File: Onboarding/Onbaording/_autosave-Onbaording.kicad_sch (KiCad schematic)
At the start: 3 parts, among them J1 Screw_Terminal_2x2.54

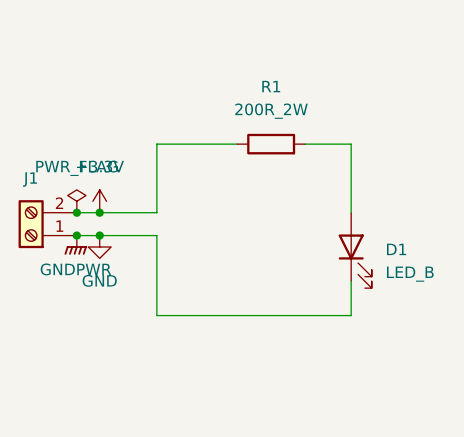
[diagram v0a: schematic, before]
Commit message: more instructions
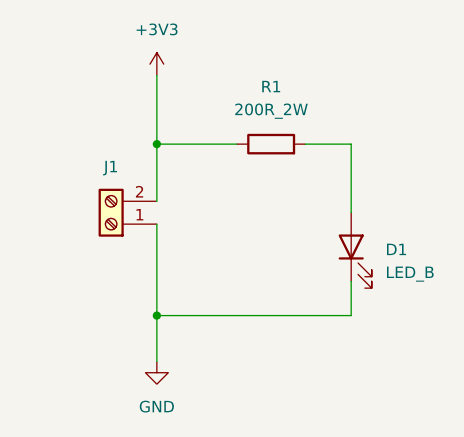
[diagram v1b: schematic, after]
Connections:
- net +3.3V renamed +3V3
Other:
- moved on the sheet: J1
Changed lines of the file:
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@@
 	(paper "A5")
 	(junction
-		(at 53.34 43.18)
+		(at 59.69 33.02)
 		(diameter 0)
 		(color 0 0 0 0)
 	)
 	(junction
-		(at 50.8 40.64)
+		(at 59.69 52.07)
 		(diameter 0)
 		(color 0 0 0 0)
 	)
-	(junction
-		(at 50.8 43.18)
-		(diameter 0)
-		(color 0 0 0 0)
-	)
-	(junction
-		(at 53.34 40.64)
-		(diameter 0)
-		(color 0 0 0 0)
-	)
 	(wire
 		(pts
@@
 	(wire
 		(pts
-			(xy 53.34 40.64) (xy 59.69 40.64)
+			(xy 59.69 41.91) (xy 59.69 52.07)
 		)
 		(stroke
@@
 	(wire
 		(pts
-			(xy 59.69 40.64) (xy 59.69 33.02)
-		)
-		(stroke
-			(width 0)
-			(type default)
-		)
-	)
-	(wire
-		(pts
-			(xy 59.69 43.18) (xy 59.69 52.07)
-		)
-		(stroke
-			(width 0)
-			(type default)
-		)
-	)
-	(wire
-		(pts
 			(xy 59.69 52.07) (xy 81.28 52.07)
 		)
@@
 	(wire
 		(pts
-			(xy 50.8 40.64) (xy 53.34 40.64)
-		)
-		(stroke
-			(width 0)
-			(type default)
-		)
-	)
-	(wire
-		(pts
-			(xy 53.34 43.18) (xy 59.69 43.18)
+			(xy 59.69 33.02) (xy 59.69 39.37)
 		)
 		(stroke
@@
 	(wire
 		(pts
-			(xy 50.8 43.18) (xy 53.34 43.18)
+			(xy 59.69 25.4) (xy 59.69 33.02)
+		)
+		(stroke
+			(width 0)
+			(type default)
+		)
+	)
+	(wire
+		(pts
+			(xy 59.69 57.15) (xy 59.69 52.07)
 		)
 		(stroke
@@
 			(width 0)
 			(type default)
-		)
-	)
-	(symbol
-		(lib_id "power:GNDPWR")
-		(at 50.8 43.18 0)
-		(unit 1)
-		(exclude_from_sim no)
-		(in_bom yes)
-		(on_board yes)
-		(dnp no)
-		(fields_autoplaced yes)
-		(property "Reference" "#PWR03"
-			(at 50.8 48.26 0)
-			(effects
-				(font
-					(size 1.27 1.27)
-				)
-				(hide yes)
-			)
-		)
-		(property "Value" "GNDPWR"
-			(at 50.673 46.99 0)
-			(effects
-				(font
-					(size 1.27 1.27)
-				)
-			)
-		)
-		(property "Footprint" ""
-			(at 50.8 44.45 0)
-			(effects
-				(font
-					(size 1.27 1.27)
-				)
-				(hide yes)
-			)
-		)
-		(property "Datasheet" ""
-			(at 50.8 44.45 0)
-			(effects
-				(font
-					(size 1.27 1.27)
-				)
-				(hide yes)
-			)
-		)
-		(property "Description" "Power symbol creates a global label with name \"GNDPWR\" , global ground"
-			(at 50.8 43.18 0)
-			(effects
-				(font
-					(size 1.27 1.27)
-				)
-				(hide yes)
-			)
-		)
-		(pin "1"
-		)
-		(instances
-			(project ""
-				(path "/e318a63f-e1fd-4a3a-bd56-00f9b3552079"
-					(reference "#PWR03")
-					(unit 1)
-				)
-			)
 		)
 	)
@@
 	(symbol
 		(lib_id "power:GND")
-		(at 53.34 43.18 0)
+		(at 59.69 57.15 0)
 		(unit 1)
 		(exclude_from_sim no)
@@
 		(fields_autoplaced yes)
 		(property "Reference" "#PWR01"
-			(at 53.34 49.53 0)
+			(at 59.69 63.5 0)
 			(effects
 				(font
@@
 		)
 		(property "Value" "GND"
-			(at 53.34 48.26 0)
+			(at 59.69 62.23 0)
 			(effects
 				(font
@@
 		)
 		(property "Footprint" ""
-			(at 53.34 43.18 0)
+			(at 59.69 57.15 0)
 			(effects
 				(font
@@
 		)
 		(property "Datasheet" ""
-			(at 53.34 43.18 0)
+			(at 59.69 57.15 0)
 			(effects
 				(font
@@
 		)
 		(property "Description" "Power symbol creates a global label with name \"GND\" , ground"
-			(at 53.34 43.18 0)
+			(at 59.69 57.15 0)
 			(effects
 				(font
@@
 		)
 		(instances
-			(project "Onbaording"
+			(project ""
 				(path "/e318a63f-e1fd-4a3a-bd56-00f9b3552079"
 					(reference "#PWR01")
@@
 	)
 	(symbol
-		(lib_id "power:PWR_FLAG")
-		(at 50.8 40.64 0)
+		(lib_id "power:+3V3")
+		(at 59.69 25.4 0)
 		(unit 1)
 		(exclude_from_sim no)
@@
 		(dnp no)
 		(fields_autoplaced yes)
-		(property "Reference" "#FLG01"
-			(at 50.8 38.735 0)
-			(effects
-				(font
-					(size 1.27 1.27)
-				)
-				(hide yes)
-			)
-		)
-		(property "Value" "PWR_FLAG"
-			(at 50.8 35.56 0)
+		(property "Reference" "#PWR02"
+			(at 59.69 29.21 0)
+			(effects
+				(font
+					(size 1.27 1.27)
+				)
+				(hide yes)
+			)
+		)
+		(property "Value" "+3V3"
+			(at 59.69 20.32 0)
 			(effects
 				(font
@@
 		)
 		(property "Footprint" ""
-			(at 50.8 40.64 0)
-			(effects
-				(font
-					(size 1.27 1.27)
-				)
-				(hide yes)
-			)
-		)
-		(property "Datasheet" "~"
-			(at 50.8 40.64 0)
-			(effects
-				(font
-					(size 1.27 1.27)
-				)
-				(hide yes)
-			)
-		)
-		(property "Description" "Special symbol for telling ERC where power comes from"
-			(at 50.8 40.64 0)
+			(at 59.69 25.4 0)
+			(effects
+				(font
+					(size 1.27 1.27)
+				)
+				(hide yes)
+			)
+		)
+		(property "Datasheet" ""
+			(at 59.69 25.4 0)
+			(effects
+				(font
+					(size 1.27 1.27)
+				)
+				(hide yes)
+			)
+		)
+		(property "Description" "Power symbol creates a global label with name \"+3V3\""
+			(at 59.69 25.4 0)
 			(effects
 				(font
@@
 			(project ""
 				(path "/e318a63f-e1fd-4a3a-bd56-00f9b3552079"
-					(reference "#FLG01")
+					(reference "#PWR02")
 					(unit 1)
 				)
@@
 	(symbol
 		(lib_id "rsx_header_screw:Screw_Terminal_2x2.54")
-		(at 45.72 43.18 180)
+		(at 54.61 41.91 180)
 		(unit 1)
 		(exclude_from_sim no)
@@
 		(fields_autoplaced yes)
 		(property "Reference" "J1"
-			(at 45.72 36.83 0)
+			(at 54.61 35.56 0)
 			(effects
 				(font
@@
 		)
 		(property "Value" "Screw_Terminal_2x2.54"
-			(at 45.72 38.1 0)
+			(at 54.61 36.83 0)
 			(effects
 				(font
@@
 		)
 		(property "Footprint" "rsx_headers_screw:Wurth_691210910002"
-			(at 45.72 43.18 0)
+			(at 54.61 41.91 0)
 			(effects
 				(font
@@
 		)
 		(property "Datasheet" "~"
-			(at 45.72 43.18 0)
+			(at 54.61 41.91 0)
 			(effects
 				(font
@@
 		)
 		(property "Description" "TERM BLOCK 2P HORIZON 2.54MM PCB"
-			(at 45.72 43.18 0)
+			(at 54.61 41.91 0)
 			(effects
 				(font
@@
 		)
 		(property "MFR" "Würth Elektronik"
-			(at 45.72 43.18 0)
+			(at 54.61 41.91 0)
 			(effects
 				(font
@@
 		)
 		(property "DPN" "732-691210910002-ND"
-			(at 45.72 43.18 0)
+			(at 54.61 41.91 0)
 			(effects
 				(font
@@
 		)
 		(property "MPN" "691210910002"
-			(at 45.72 43.18 0)
+			(at 54.61 41.91 0)
 			(effects
 				(font
@@
 					(unit 1)
 				)
-			)
-		)
-	)
-	(symbol
-		(lib_id "power:+3.3V")
-		(at 53.34 40.64 0)
-		(unit 1)
-		(exclude_from_sim no)
-		(in_bom yes)
-		(on_board yes)
-		(dnp no)
-		(fields_autoplaced yes)
-		(property "Reference" "#PWR02"
-			(at 53.34 44.45 0)
-			(effects
-				(font
-					(size 1.27 1.27)
-				)
-				(hide yes)
-			)
-		)
-		(property "Value" "+3.3V"
-			(at 53.34 35.56 0)
-			(effects
-				(font
-					(size 1.27 1.27)
-				)
-			)
-		)
-		(property "Footprint" ""
-			(at 53.34 40.64 0)
-			(effects
-				(font
-					(size 1.27 1.27)
-				)
-				(hide yes)
-			)
-		)
-		(property "Datasheet" ""
-			(at 53.34 40.64 0)
-			(effects
-				(font
-					(size 1.27 1.27)
-				)
-				(hide yes)
-			)
-		)
-		(property "Description" "Power symbol creates a global label with name \"+3.3V\""
-			(at 53.34 40.64 0)
-			(effects
-				(font
-					(size 1.27 1.27)
-				)
-				(hide yes)
-			)
-		)
-		(pin "1"
-		)
-		(instances
-			(project ""
-				(path "/e318a63f-e1fd-4a3a-bd56-00f9b3552079"
-					(reference "#PWR02")
-					(unit 1)
-				)
